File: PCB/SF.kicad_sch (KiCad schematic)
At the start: 27 parts, among them SW1 SW_Push, SW2 SW_Push, SW3 SW_Push, SW4 SW_Push, SW5 SW_Push, SW6 SW_Push, SW7 SW_Push, SW8 SW_Push, U1 XIAO-RP2040-DIP

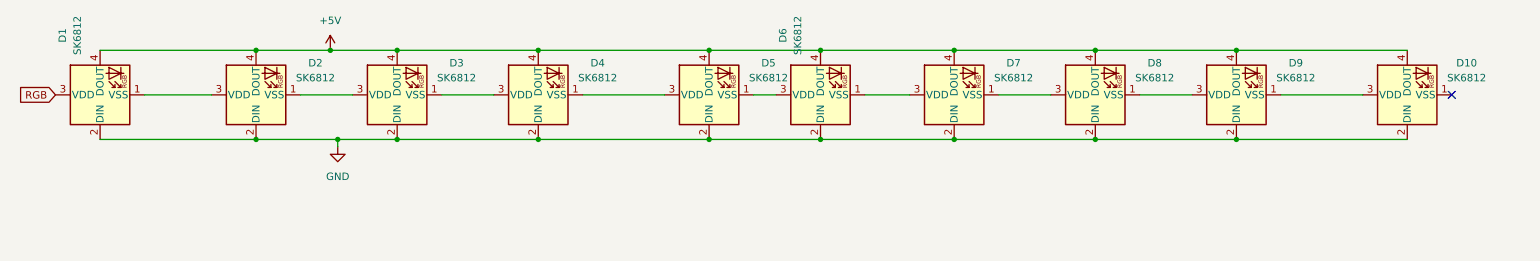
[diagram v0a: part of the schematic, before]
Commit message: Add files via upload
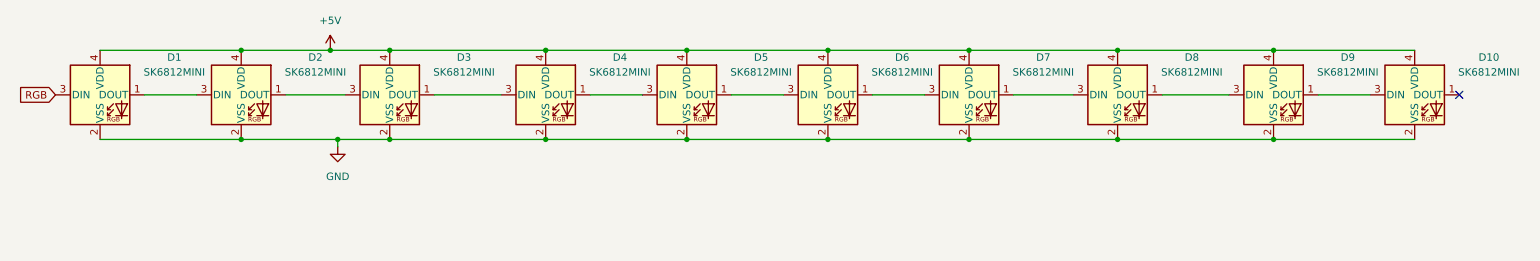
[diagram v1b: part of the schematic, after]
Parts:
- removed D1, D10, D2, D3, D4, D5, D6, D7, D8, D9: SK6812, LED_SMD:LED_SK6812MINI_PLCC4_3.5x3.5mm_P1.75mm, symbol LED:SK6812
- added D1, D10, D2, D3, D4, D5, D6, D7, D8, D9: SK6812MINI, LED_SMD:LED_SK6812MINI_PLCC4_3.5x3.5mm_P1.75mm, symbol LED:SK6812MINI
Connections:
- net +5V: now also D1.4 (VDD), D10.4 (VDD), D2.4 (VDD), D3.4 (VDD), D4.4 (VDD), D5.4 (VDD), D6.4 (VDD), D7.4 (VDD), D8.4 (VDD), D9.4 (VDD)
- net GND: now also D1.2 (VSS), D10.2 (VSS), D2.2 (VSS), D3.2 (VSS), D4.2 (VSS), D5.2 (VSS), D6.2 (VSS), D7.2 (VSS), D8.2 (VSS), D9.2 (VSS)
- net RGB: now also D1.3 (DIN)
- new net: D8.1 (DOUT), D9.3 (DIN)
- new net: D7.1 (DOUT), D8.3 (DIN)
- new net: D2.1 (DOUT), D3.3 (DIN)
- new net: D1.1 (DOUT), D2.3 (DIN)
- new net: D10.3 (DIN), D9.1 (DOUT)
- new net: D3.1 (DOUT), D4.3 (DIN)
- new net: D6.1 (DOUT), D7.3 (DIN)
- new net: D5.1 (DOUT), D6.3 (DIN)
- new net: D4.1 (DOUT), D5.3 (DIN)
